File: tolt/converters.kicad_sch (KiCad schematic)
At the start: 41 parts, among them U14 AMS1117-3.3, U15 LP5907MFX-3.3, U16 TPS62173DSG, U19 TLV61047DDC, U24 PQDE6W-Q110 / RD5-110S12W

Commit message: modified:   tolt/conn.kicad_sch 	modified:   tolt/converters.kicad_sch 	modified:   tolt/inter.kicad_sch 	modified:   tolt/powerstage.kicad_sch 	modified:   tolt/stm32.kicad_sch 	modified:   tolt/tolt.kicad_pcb 	modified:   tolt/tolt.kicad_pro
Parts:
- C62, C64, C66, C67, C69: footprint Capacitor_SMD:C_0402_1005Metric_Pad0.74x0.62mm_HandSolder -> Capacitor_SMD:C_0402_1005Metric
- C63, C65, C68, C70, C71, C72, C73, C74, C75, C76, C77, C85: footprint Capacitor_SMD:C_1210_3225Metric_Pad1.33x2.70mm_HandSolder -> Capacitor_SMD:C_1210_3225Metric
- R94, R95: footprint Resistor_SMD:R_0603_1608Metric_Pad0.98x0.95mm_HandSolder -> Resistor_SMD:R_0603_1608Metric
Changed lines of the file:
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@@
 			)
 		)
-		(property "Footprint" "Capacitor_SMD:C_1210_3225Metric_Pad1.33x2.70mm_HandSolder"
+		(property "Footprint" "Capacitor_SMD:C_1210_3225Metric"
 			(at 63.7032 94.234 0)
 			(effects
@@
 			)
 		)
-		(property "Footprint" "Capacitor_SMD:C_0402_1005Metric_Pad0.74x0.62mm_HandSolder"
+		(property "Footprint" "Capacitor_SMD:C_0402_1005Metric"
 			(at 51.2572 94.234 0)
 			(effects
@@
 			)
 		)
-		(property "Footprint" "Capacitor_SMD:C_0402_1005Metric_Pad0.74x0.62mm_HandSolder"
+		(property "Footprint" "Capacitor_SMD:C_0402_1005Metric"
 			(at 90.8812 94.234 0)
 			(effects
@@
 			)
 		)
-		(property "Footprint" "Capacitor_SMD:C_0402_1005Metric_Pad0.74x0.62mm_HandSolder"
+		(property "Footprint" "Capacitor_SMD:C_0402_1005Metric"
 			(at 52.5272 135.382 0)
 			(effects
@@
 			)
 		)
-		(property "Footprint" "Resistor_SMD:R_0603_1608Metric_Pad0.98x0.95mm_HandSolder"
+		(property "Footprint" "Resistor_SMD:R_0603_1608Metric"
 			(at 221.996 46.482 90)
 			(effects
@@
 			)
 		)
-		(property "Footprint" "Capacitor_SMD:C_1210_3225Metric_Pad1.33x2.70mm_HandSolder"
+		(property "Footprint" "Capacitor_SMD:C_1210_3225Metric"
 			(at 103.6828 35.306 0)
 			(effects
@@
 			)
 		)
-		(property "Footprint" "Capacitor_SMD:C_0402_1005Metric_Pad0.74x0.62mm_HandSolder"
+		(property "Footprint" "Capacitor_SMD:C_0402_1005Metric"
 			(at 92.4052 135.382 0)
 			(effects
@@
 			)
 		)
-		(property "Footprint" "Capacitor_SMD:C_1210_3225Metric_Pad1.33x2.70mm_HandSolder"
+		(property "Footprint" "Capacitor_SMD:C_1210_3225Metric"
 			(at 247.1928 123.952 0)
 			(effects
@@
 			)
 		)
-		(property "Footprint" "Capacitor_SMD:C_1210_3225Metric_Pad1.33x2.70mm_HandSolder"
+		(property "Footprint" "Capacitor_SMD:C_1210_3225Metric"
 			(at 236.5248 123.952 0)
 			(effects
@@
 			)
 		)
-		(property "Footprint" "Capacitor_SMD:C_1210_3225Metric_Pad1.33x2.70mm_HandSolder"
+		(property "Footprint" "Capacitor_SMD:C_1210_3225Metric"
 			(at 183.4388 44.704 0)
 			(effects
@@
 			)
 		)
-		(property "Footprint" "Capacitor_SMD:C_1210_3225Metric_Pad1.33x2.70mm_HandSolder"
+		(property "Footprint" "Capacitor_SMD:C_1210_3225Metric"
 			(at 104.8512 135.382 0)
 			(effects
@@
 			)
 		)
-		(property "Footprint" "Capacitor_SMD:C_1210_3225Metric_Pad1.33x2.70mm_HandSolder"
+		(property "Footprint" "Capacitor_SMD:C_1210_3225Metric"
 			(at 39.1668 34.29 0)
 			(effects
@@
 			)
 		)
-		(property "Footprint" "Capacitor_SMD:C_1210_3225Metric_Pad1.33x2.70mm_HandSolder"
+		(property "Footprint" "Capacitor_SMD:C_1210_3225Metric"
 			(at 245.9228 40.132 0)
 			(effects
@@
 			)
 		)
-		(property "Footprint" "Capacitor_SMD:C_1210_3225Metric_Pad1.33x2.70mm_HandSolder"
+		(property "Footprint" "Capacitor_SMD:C_1210_3225Metric"
 			(at 256.8448 40.132 0)
 			(effects
@@
 			)
 		)
-		(property "Footprint" "Capacitor_SMD:C_1210_3225Metric_Pad1.33x2.70mm_HandSolder"
+		(property "Footprint" "Capacitor_SMD:C_1210_3225Metric"
 			(at 64.9732 135.382 0)
 			(effects
@@
 			)
 		)
-		(property "Footprint" "Resistor_SMD:R_0603_1608Metric_Pad0.98x0.95mm_HandSolder"
+		(property "Footprint" "Resistor_SMD:R_0603_1608Metric"
 			(at 221.996 54.102 90)
 			(effects
@@
 			)
 		)
-		(property "Footprint" "Capacitor_SMD:C_1210_3225Metric_Pad1.33x2.70mm_HandSolder"
+		(property "Footprint" "Capacitor_SMD:C_1210_3225Metric"
 			(at 103.3272 94.234 0)
 			(effects
@@
 			)
 		)
-		(property "Footprint" "Capacitor_SMD:C_0402_1005Metric_Pad0.74x0.62mm_HandSolder"
+		(property "Footprint" "Capacitor_SMD:C_0402_1005Metric"
 			(at 117.8052 135.382 0)
 			(effects
@@
 			)
 		)
-		(property "Footprint" "Capacitor_SMD:C_1210_3225Metric_Pad1.33x2.70mm_HandSolder"
+		(property "Footprint" "Capacitor_SMD:C_1210_3225Metric"
 			(at 93.0148 35.306 0)
 			(effects

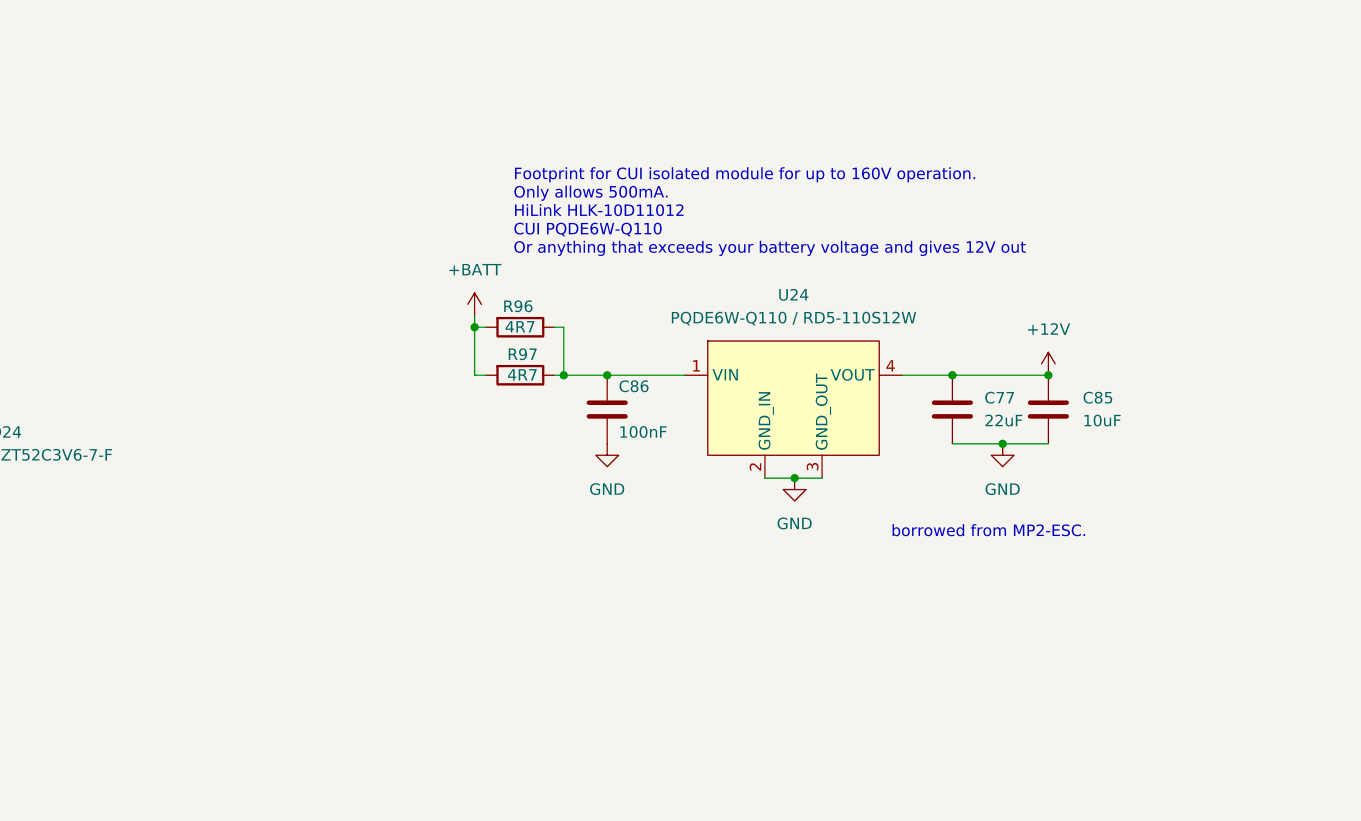
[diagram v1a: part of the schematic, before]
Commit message: ltc
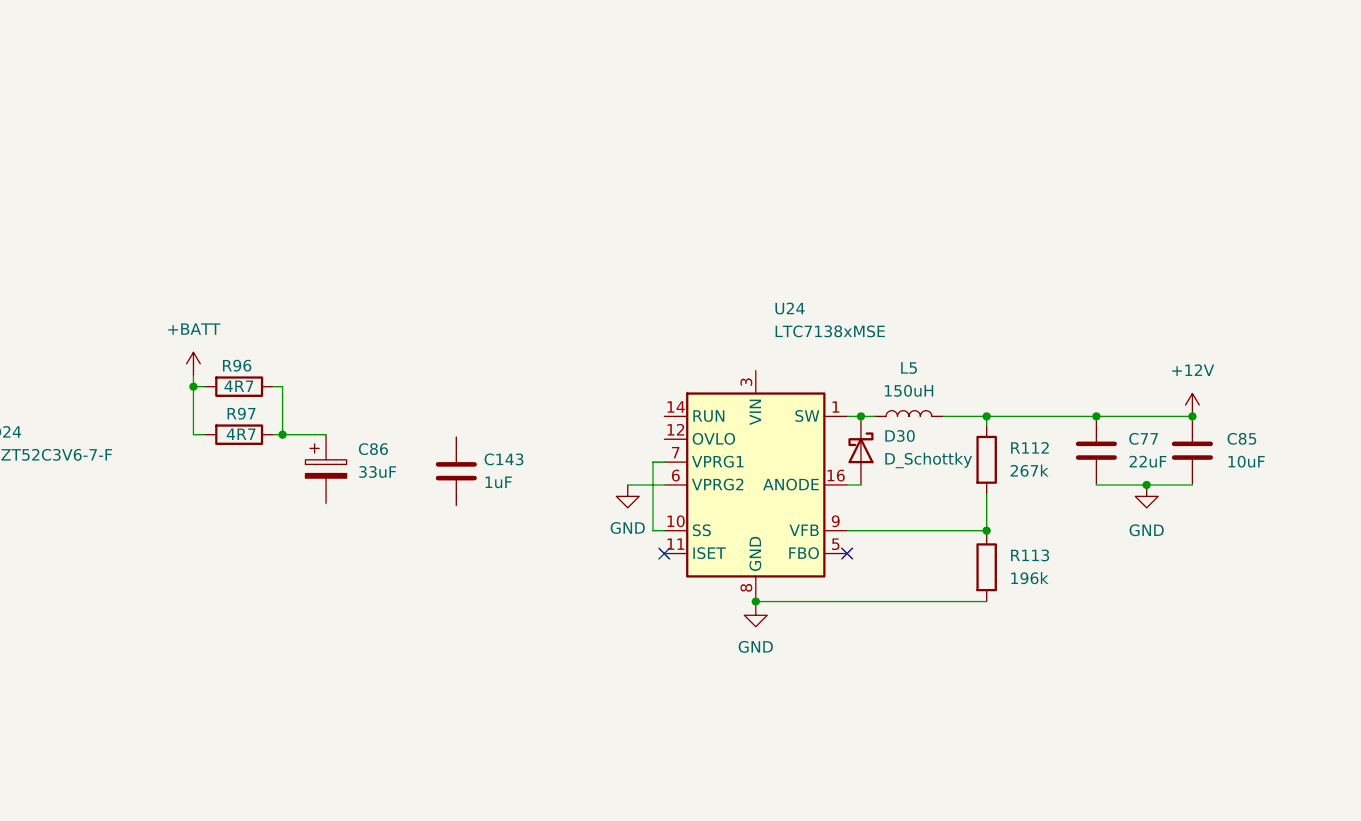
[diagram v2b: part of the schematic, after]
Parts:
- removed C86: 100nF, Capacitor_SMD:C_0805_2012Metric, symbol Device:C
- removed U24: PQDE6W-Q110 / RD5-110S12W, Library:PQDE6W, symbol CCC_ESC_Custom_Symbols:PQDE6W-Q110
- added C143: 1uF, symbol Device:C
- added C86: 33uF, symbol Device:C_Polarized
- added D30: D_Schottky, symbol Device:D_Schottky
- added L5: 150uH, symbol Device:L
- added R112: 267k, symbol Device:R
- added R113: 196k, symbol Device:R
- added U24: LTC7138xMSE, Package_SO:Analog_MSOP-12-16-1EP_3x4.039mm_P0.5mm_EP1.651x2.845mm, symbol Regulator_Switching:LTC7138xMSE
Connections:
- net +12V: now also L5.2, R112.1
- net GND: now also R113.2, U24.17 (GND), U24.6 (VPRG2), U24.8 (GND)
- net at R96.1, R97.1: now also C86.1
- new net: D30.1 (K), L5.1, U24.1 (SW)
- new net: U24.10 (SS), U24.7 (VPRG1)
- new net: D30.2 (A), U24.16 (ANODE)
- new net: R112.2, R113.1, U24.9 (VFB)
- no-connect marks 0 -> 2
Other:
- note removed: "Footprint for CUI isolated module for up to 160V operation. Only allows 500mA. HiLink HLK-10D11012 CUI PQDE6W-Q110 Or anything that exceeds your battery voltage and gives 12V out"
- note removed: "borrowed from MP2-ESC."
- moved on the sheet: C77, C85, R96, R97

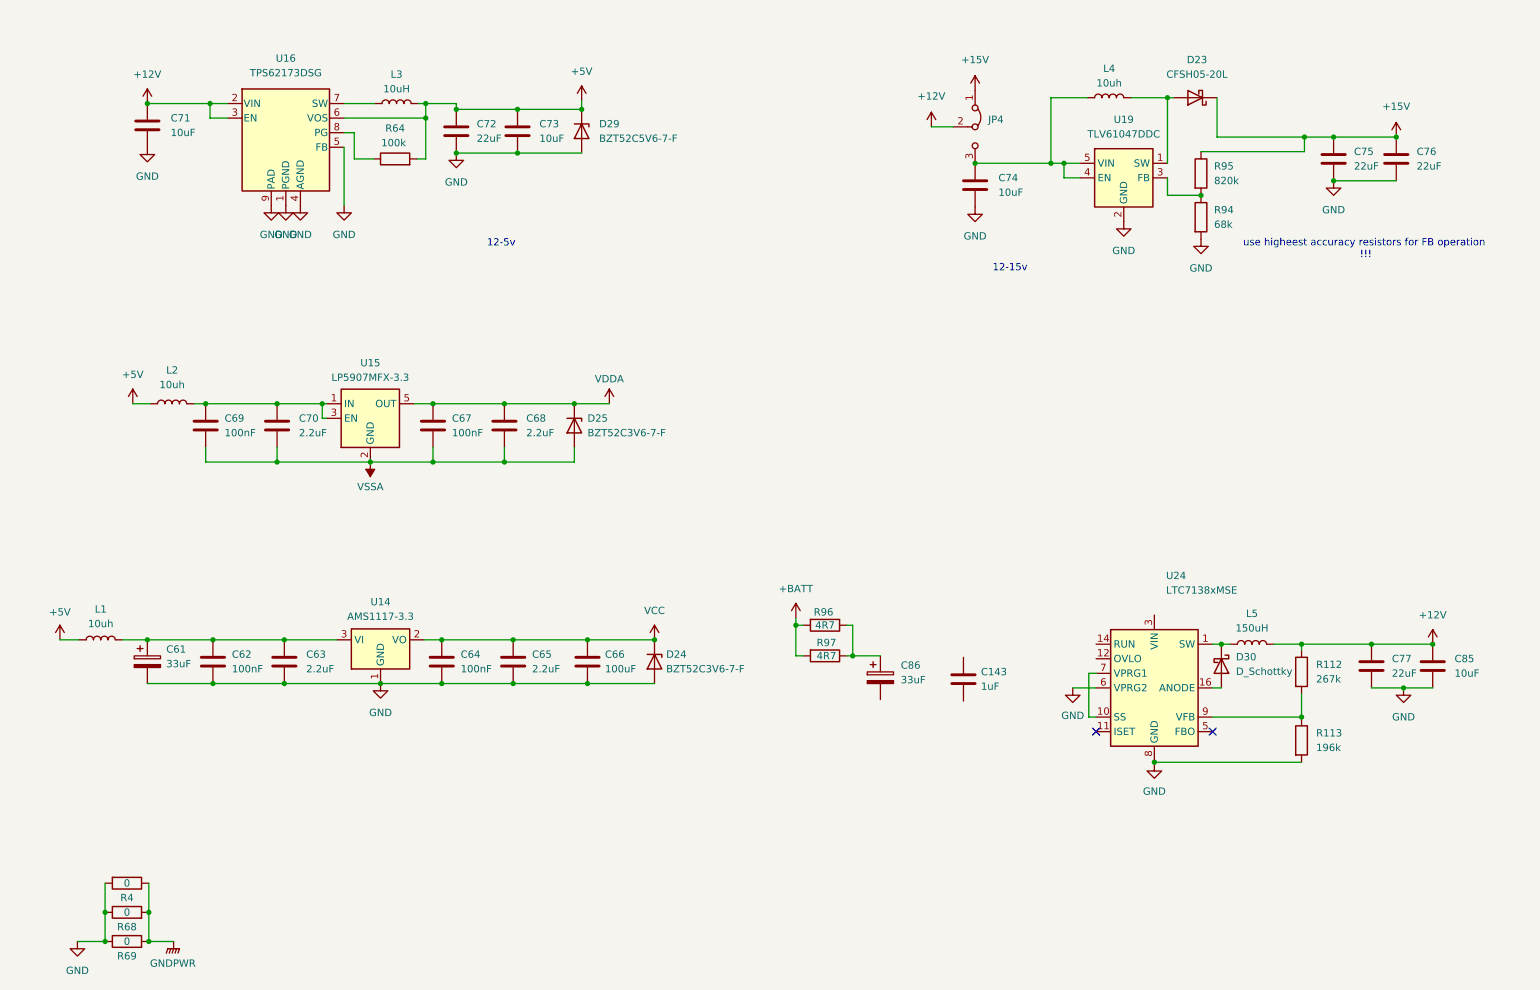
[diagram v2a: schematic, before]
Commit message: a
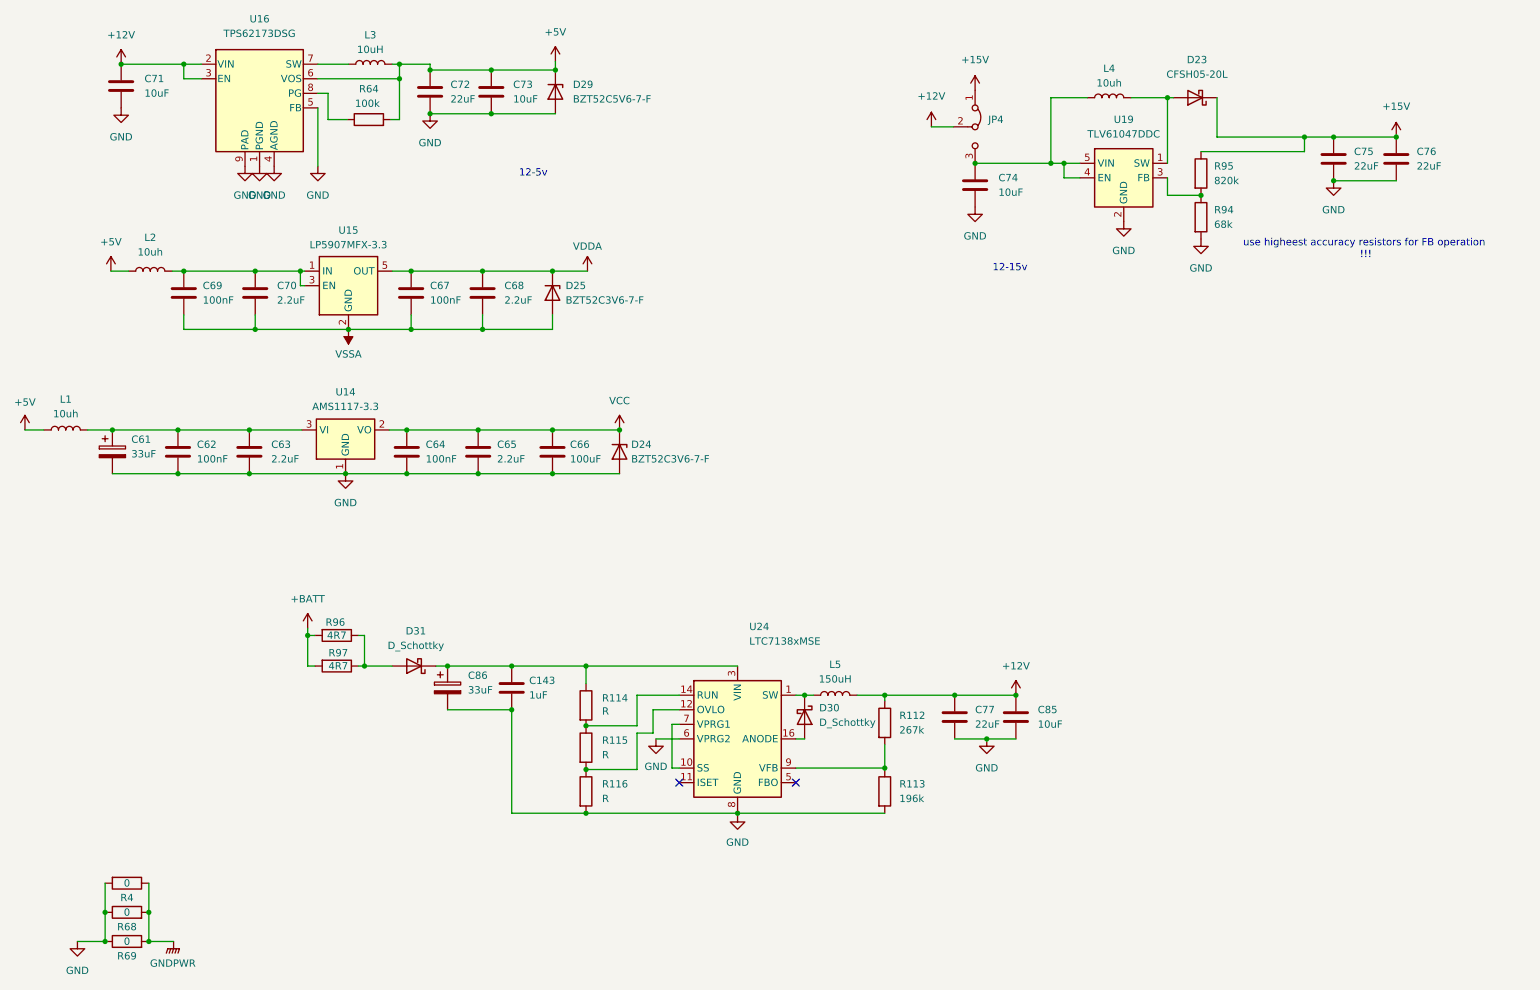
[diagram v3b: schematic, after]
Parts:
- added D31: D_Schottky, symbol Device:D_Schottky
- added R114, R115, R116: R, symbol Device:R
- C143: footprint (none) -> Capacitor_SMD:C_2220_5750Metric
- C86: footprint (none) -> Capacitor_Tantalum_SMD:CP_EIA-3528-15_AVX-H
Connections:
- net GND: now also C143.2, C86.2, R116.2
- net at U24.12 (OVLO): now also R115.2, R116.1
- net at U24.14 (RUN): now also R114.2, R115.1
- net at U24.3 (VIN): now also C143.1, C86.1, D31.1 (K), R114.1
- net at R96.1, R97.1: now also D31.2 (A); no longer C86.1
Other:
- moved on the sheet: C143, C61, C62, C63, C64, C65, C66, C67, C68, C69, C70, C71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
